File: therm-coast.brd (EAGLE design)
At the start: 33 x 33 mm, 19 parts, among them U1 ATTINY85-20SU

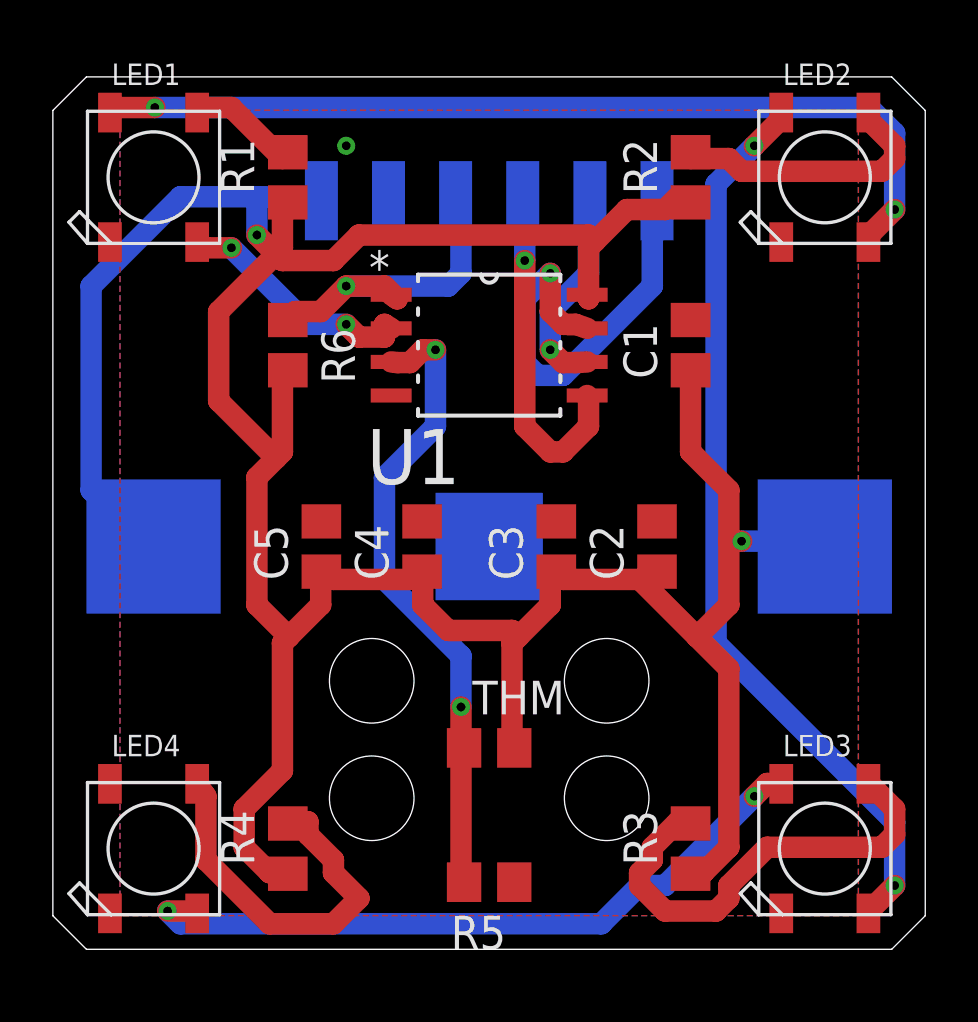
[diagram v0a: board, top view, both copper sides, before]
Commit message: Rev 1.0
Better Route and Placement, Silks
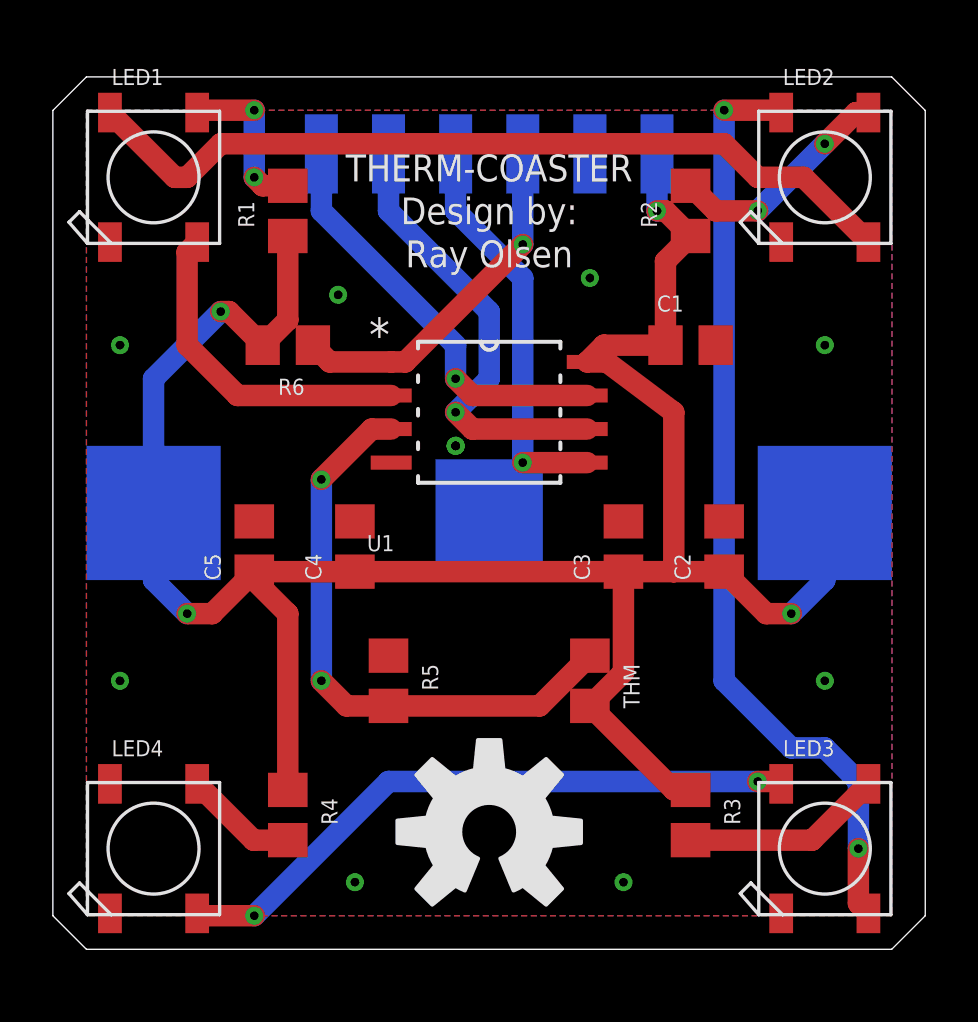
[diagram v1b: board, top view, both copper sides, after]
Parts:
- added LOGO1: OSHW-LOGOL, SparkFun-Aesthetics:OSHW-LOGO-L
- moved R5 8.52 mm to (12.7, 10.2), turned to 270 degrees
- moved J1 5.08 mm to (16.5, 26.7), turned to 0 degrees
- moved THM 4.58 mm to (20.3, 10.2), turned to 270 degrees
- moved C4 2.54 mm to (11.4, 15.2)
- moved C5 2.54 mm to (7.62, 15.2)
- moved C2 2.54 mm to (25.4, 15.2)
- moved C3 2.54 mm to (21.6, 15.2)
- moved U1 2.54 mm to (16.5, 20.3)
- moved BT1 1.27 mm to (16.5, 16.5)
- moved R3 1.27 mm to (24.1, 5.08), turned to 270 degrees
- moved R4 1.27 mm to (8.89, 5.08), turned to 270 degrees
- moved R1 1.27 mm to (8.89, 27.9)
- moved R2 1.27 mm to (24.1, 27.9)
- turned C1 to 0 degrees
- turned R6 to 180 degrees
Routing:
- net VCC: track 129.6 -> 88.9 mm, vias 2 -> 4
- net N$4: track 14.6 -> 4.31 mm
- net N$3: track 17.5 -> 7.61 mm
- net MISO: track 7.84 -> 17.1 mm
- net LED_DATA: track 9.33 -> 12.6 mm, vias 2 -> 0
- net N$5: track 34.7 -> 31.8 mm, vias 2 -> 0
- net N$7: track 26.8 -> 24.3 mm
- net MOSI/SDA: track 12.9 -> 15.2 mm
- net N$2: track 10.5 -> 8.66 mm, vias 0 -> 2
- net N$1: track 4.39 -> 6.14 mm, vias 0 -> 2
- net TEMP: track 24.1 -> 22.4 mm
- net N$6: track 34.5 -> 35.6 mm
- net RESET: track 12.5 -> 13.5 mm
- net SCK/SCL: track 16.5 -> 15.9 mm
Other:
- board text added: "THERM-COASTER Design by: Ray Olsen"
